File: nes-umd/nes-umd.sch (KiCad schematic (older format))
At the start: 2 parts, among them CON101 NES-CONN, CON102 UMD-CONN

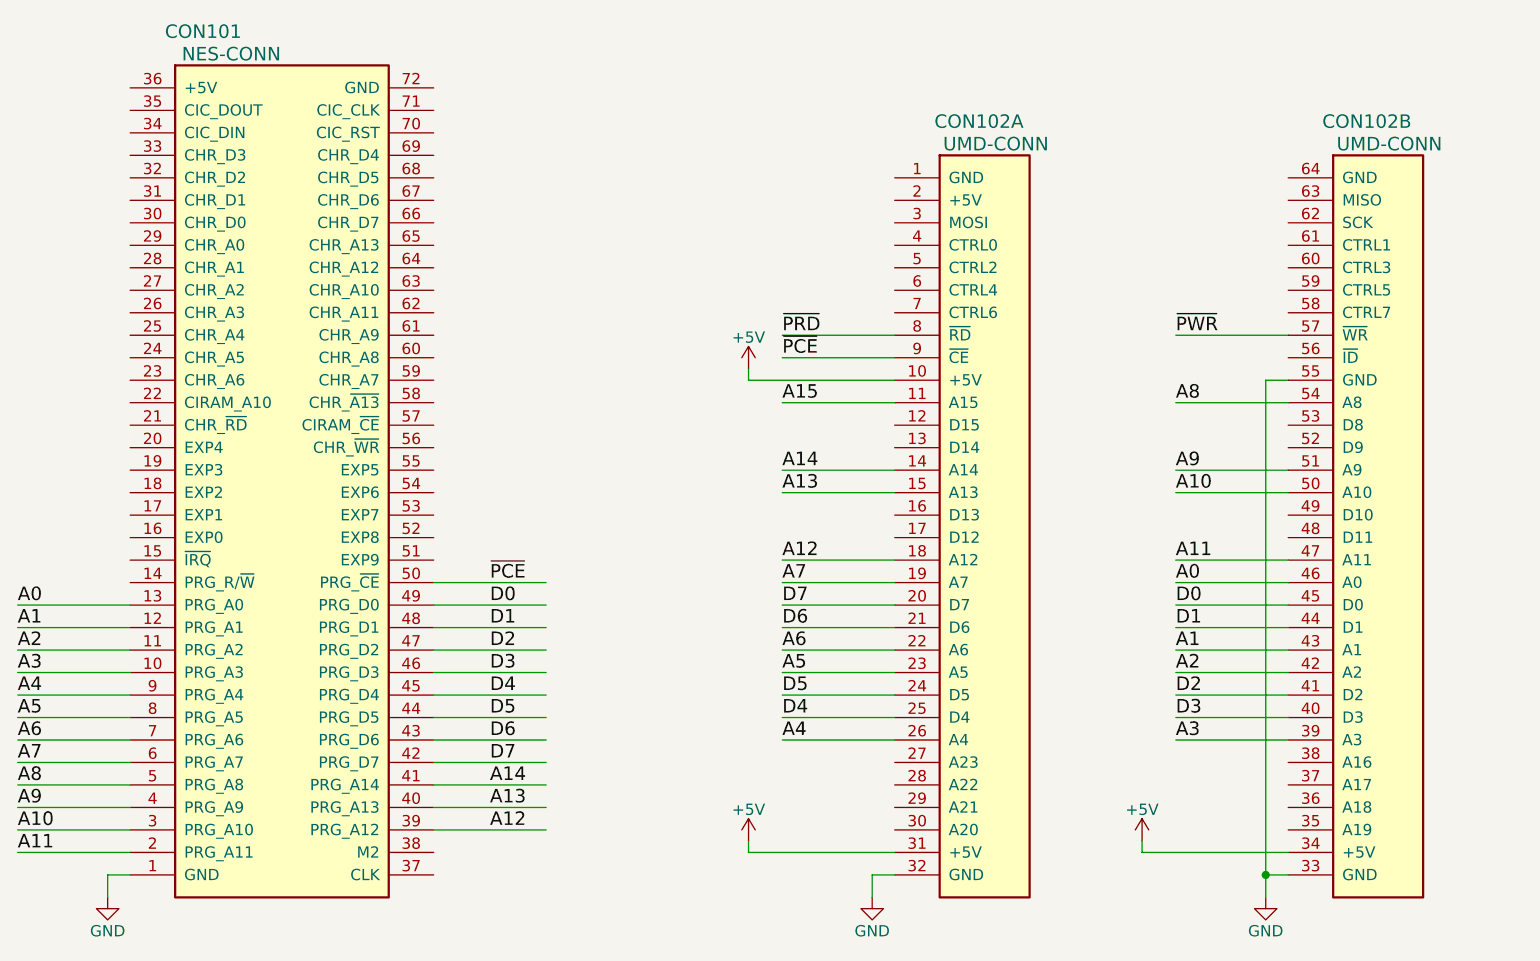
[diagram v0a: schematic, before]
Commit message: schematic work
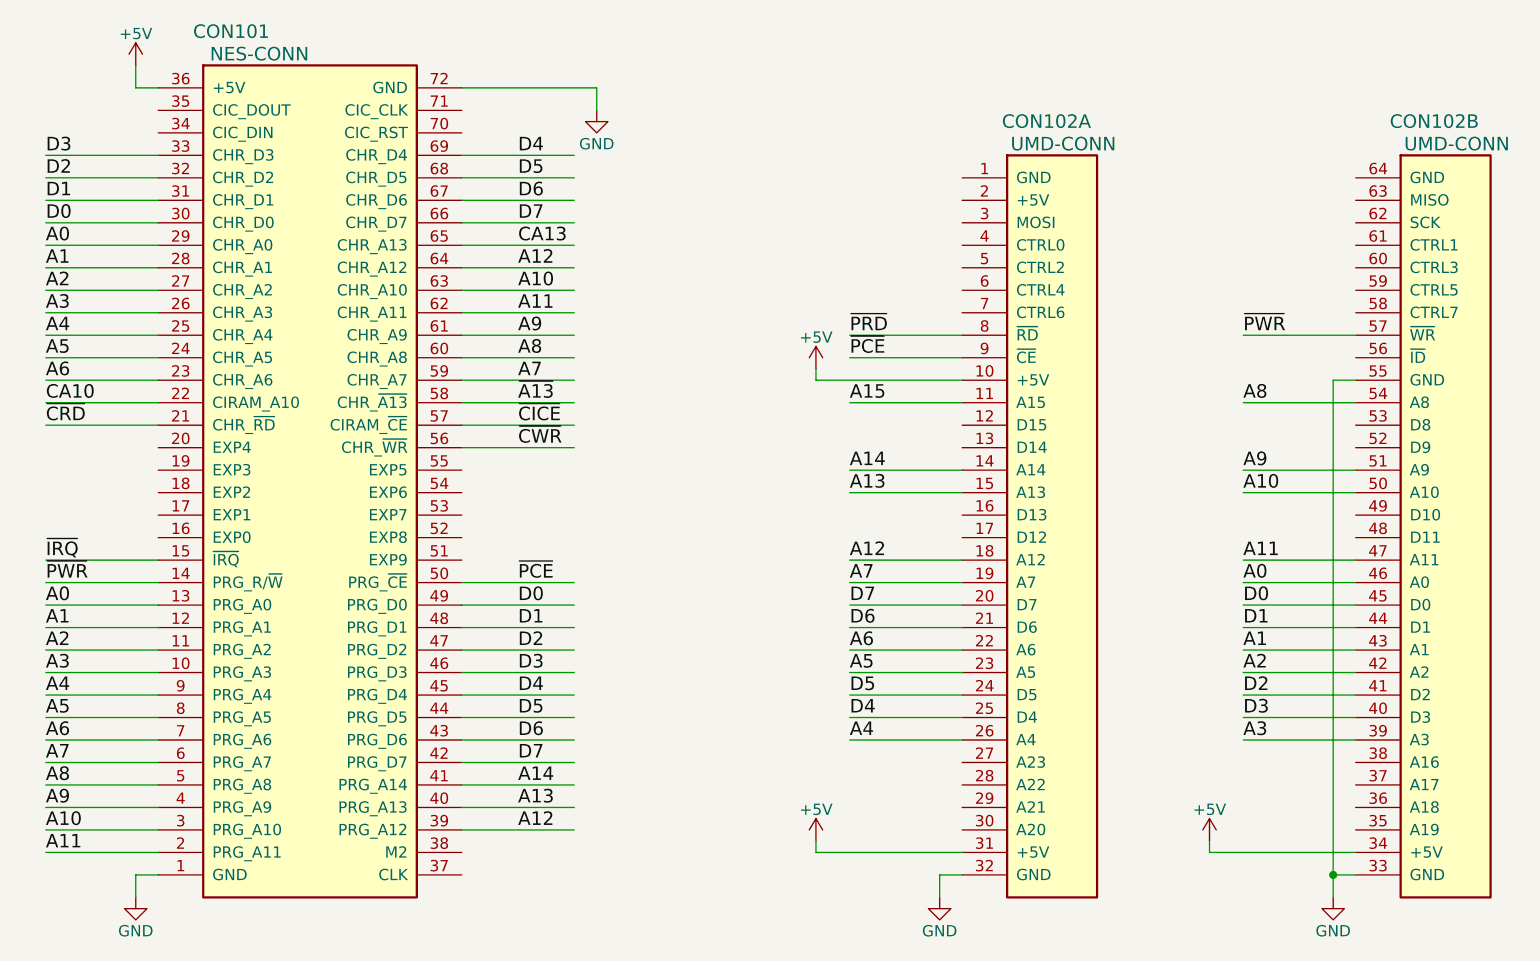
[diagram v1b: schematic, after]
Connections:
- net labels added: CA10, CA13, ~A13, ~CICE, ~CRD, ~CWR, ~IRQ
- wire segments 64 -> 97
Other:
- moved on the sheet: CON101, CON102A, CON102B
